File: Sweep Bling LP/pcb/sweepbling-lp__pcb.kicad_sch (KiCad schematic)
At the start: 46 parts, among them SW1 SW_Push, SW10 SW_Push, SW10_r1 SW_Push, SW11 SW_Push, SW11_r1 SW_Push, SW12 SW_Push, SW12_r1 SW_Push, SW13 SW_Push, SW13_r1 SW_Push, SW14 SW_Push, SW14_r1 SW_Push, SW15 SW_Push, SW15_r1 SW_Push, SW16 SW_Push, SW16_r1 SW_Push, SW17 SW_Push, SW17_r1 SW_Push, SW1_r1 SW_Push, SW2 SW_Push, SW2_r1 SW_Push, SW3 SW_Push, SW3_r1 SW_Push, SW4 SW_Push, SW4_r1 SW_Push, SW5 SW_Push, SW5_r1 SW_Push, SW6 SW_Push, SW6_r1 SW_Push, SW7 SW_Push, SW7_r1 SW_Push, SW8 SW_Push, SW8_r1 SW_Push, SW9 SW_Push, SW9_r1 SW_Push, U1 ProMicro-kbd, U2 ProMicro-kbd

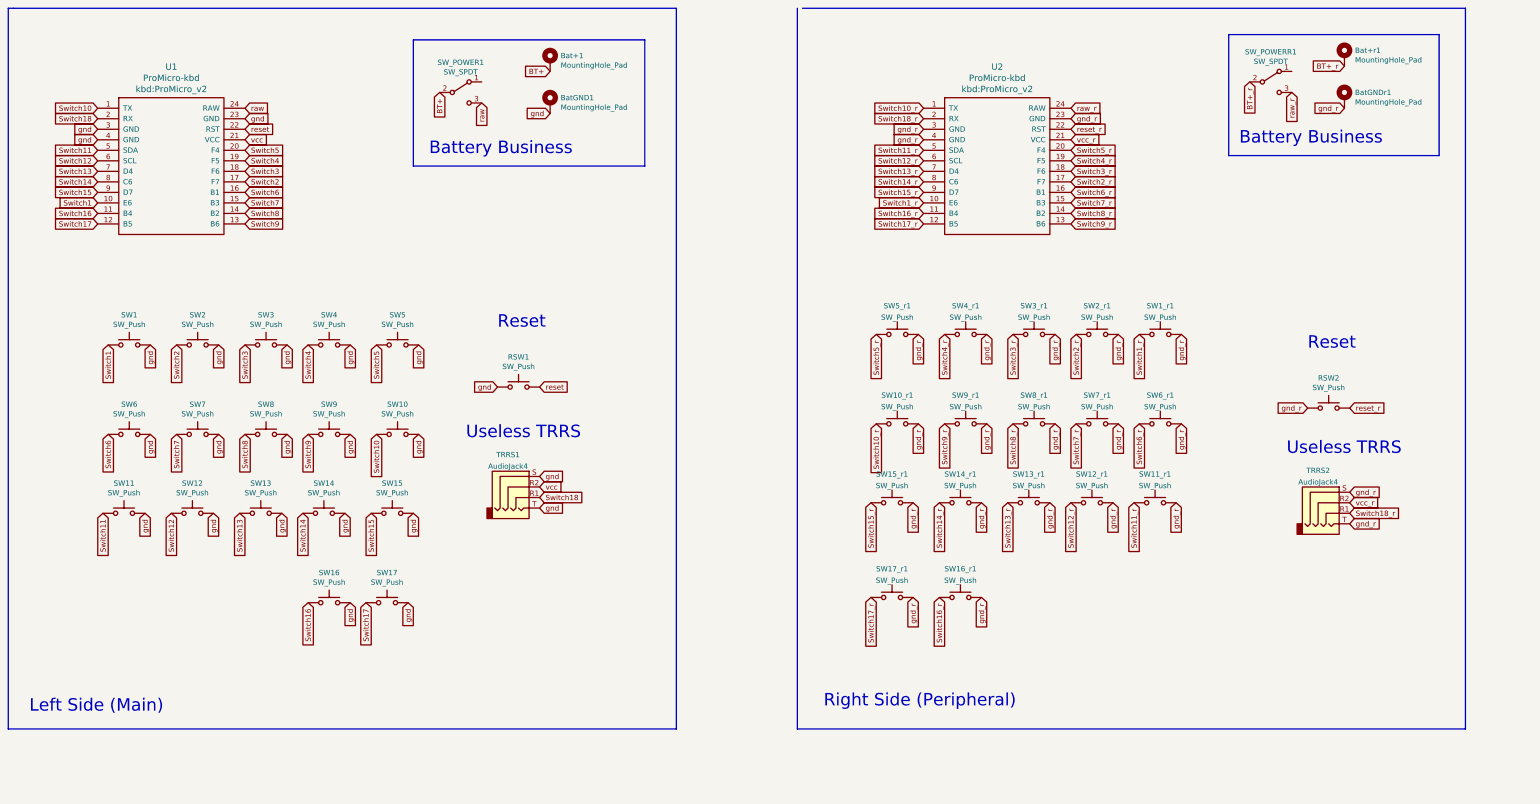
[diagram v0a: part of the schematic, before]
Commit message: made sweep bling LP Choc v2
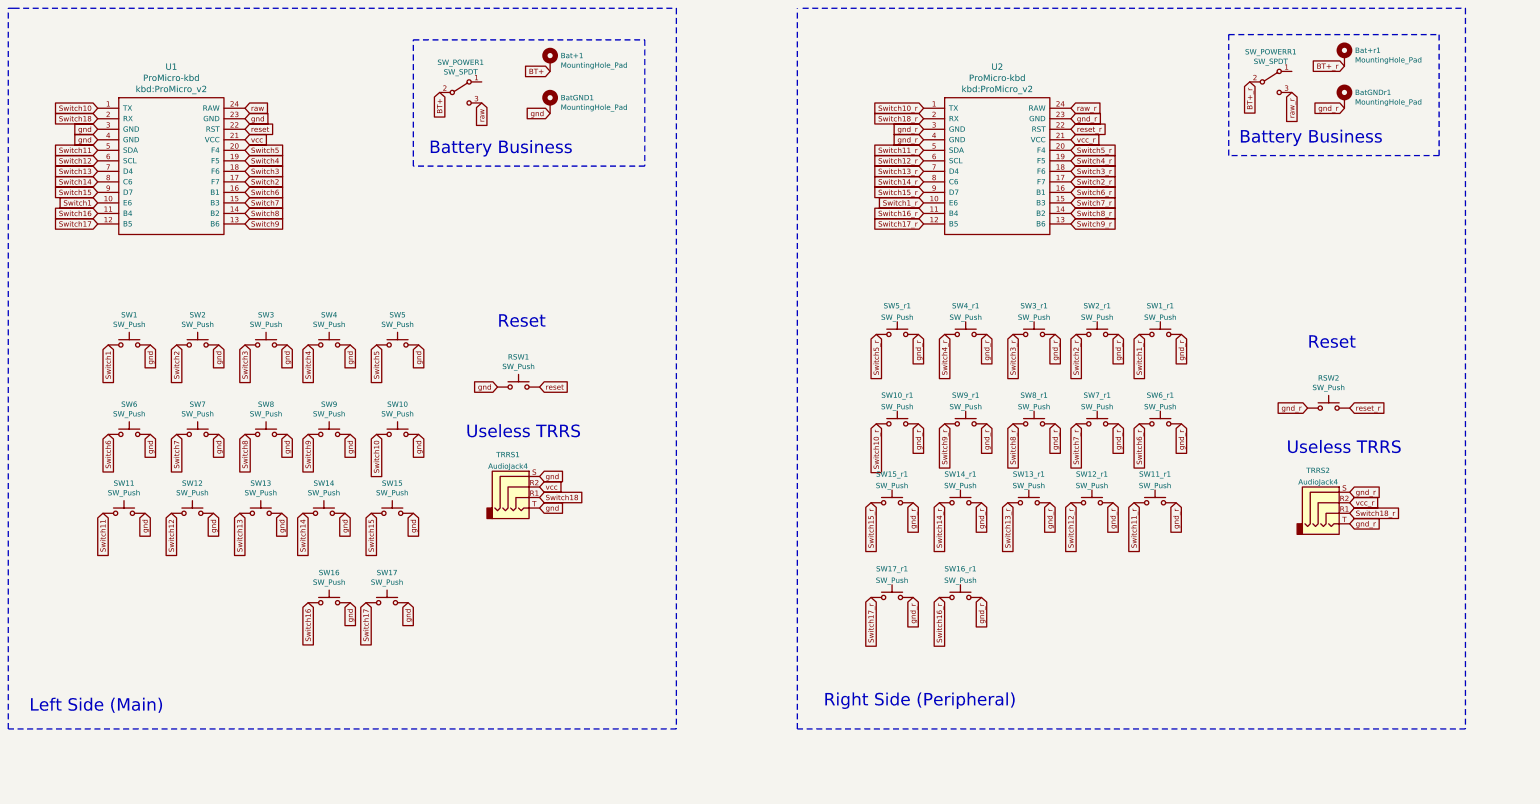
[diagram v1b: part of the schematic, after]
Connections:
- net Switch1: now also SW1.2; no longer SW1.1
- net Switch10: now also SW10.2; no longer SW10.1
- net Switch10_r: now also SW10_r1.2; no longer SW10_r1.1
- net Switch11: now also SW11.2; no longer SW11.1
- net Switch11_r: now also SW11_r1.2; no longer SW11_r1.1
- net Switch12: now also SW12.2; no longer SW12.1
- net Switch12_r: now also SW12_r1.2; no longer SW12_r1.1
- net Switch13: now also SW13.2; no longer SW13.1
- net Switch13_r: now also SW13_r1.2; no longer SW13_r1.1
- net Switch14: now also SW14.2; no longer SW14.1
- net Switch14_r: now also SW14_r1.2; no longer SW14_r1.1
- net Switch15: now also SW15.2; no longer SW15.1
- net Switch15_r: now also SW15_r1.2; no longer SW15_r1.1
- net Switch16: now also SW16.2; no longer SW16.1
- net Switch16_r: now also SW16_r1.2; no longer SW16_r1.1
- net Switch17: now also SW17.2; no longer SW17.1
- net Switch17_r: now also SW17_r1.2; no longer SW17_r1.1
- net Switch1_r: now also SW1_r1.2; no longer SW1_r1.1
- net Switch2: now also SW2.2; no longer SW2.1
- net Switch2_r: now also SW2_r1.2; no longer SW2_r1.1
- net Switch3: now also SW3.2; no longer SW3.1
- net Switch3_r: now also SW3_r1.2; no longer SW3_r1.1
- net Switch4: now also SW4.2; no longer SW4.1
- net Switch4_r: now also SW4_r1.2; no longer SW4_r1.1
- net Switch5: now also SW5.2; no longer SW5.1
- net Switch5_r: now also SW5_r1.2; no longer SW5_r1.1
- net Switch6: now also SW6.2; no longer SW6.1
- net Switch6_r: now also SW6_r1.2; no longer SW6_r1.1
- net Switch7: now also SW7.2; no longer SW7.1
- net Switch7_r: now also SW7_r1.2; no longer SW7_r1.1
- net Switch8: now also SW8.2; no longer SW8.1
- net Switch8_r: now also SW8_r1.2; no longer SW8_r1.1
- net Switch9: now also SW9.2; no longer SW9.1
- net Switch9_r: now also SW9_r1.2; no longer SW9_r1.1
- net gnd: now also SW1.1, SW10.1, SW11.1, SW12.1, SW13.1, SW14.1, SW15.1, SW16.1, SW17.1, SW2.1, SW3.1, SW4.1, SW5.1, SW6.1, SW7.1, SW8.1, SW9.1; no longer SW1.2, SW10.2, SW11.2, SW12.2, SW13.2, SW14.2, SW15.2, SW16.2, SW17.2, SW2.2, SW3.2, SW4.2, SW5.2, SW6.2, SW7.2, SW8.2, SW9.2
- net gnd_r: now also SW10_r1.1, SW11_r1.1, SW12_r1.1, SW13_r1.1, SW14_r1.1, SW15_r1.1, SW16_r1.1, SW17_r1.1, SW1_r1.1, SW2_r1.1, SW3_r1.1, SW4_r1.1, SW5_r1.1, SW6_r1.1, SW7_r1.1, SW8_r1.1, SW9_r1.1; no longer SW10_r1.2, SW11_r1.2, SW12_r1.2, SW13_r1.2, SW14_r1.2, SW15_r1.2, SW16_r1.2, SW17_r1.2, SW1_r1.2, SW2_r1.2, SW3_r1.2, SW4_r1.2, SW5_r1.2, SW6_r1.2, SW7_r1.2, SW8_r1.2, SW9_r1.2
